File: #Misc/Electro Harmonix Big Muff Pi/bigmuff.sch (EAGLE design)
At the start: 33 parts, among them IC1 TL082CP, Q1 2N7000, Q2 2N7000

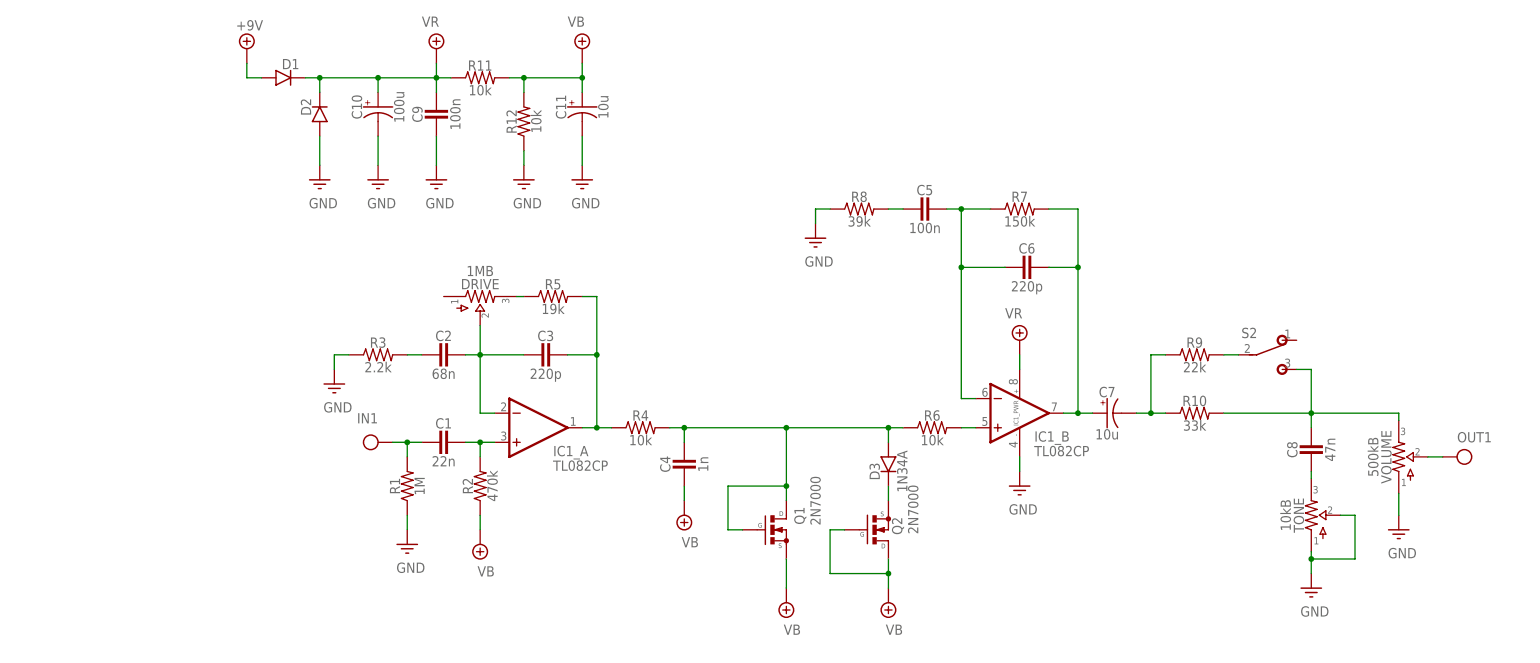
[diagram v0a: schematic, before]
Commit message: 20200322/09:12
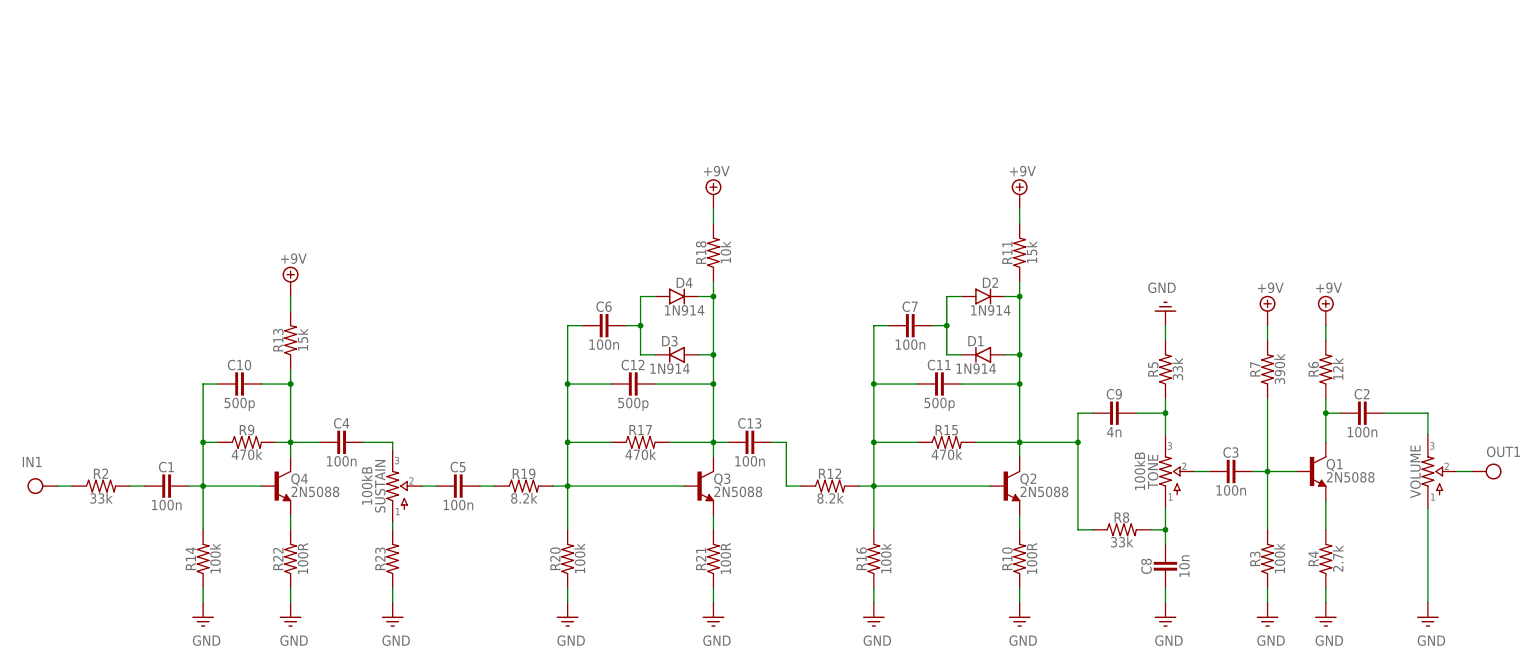
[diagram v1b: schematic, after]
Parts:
- removed DRIVE: 1MB, pedals-potentiometers:POTS16MM
- removed IC1: TL082CP, pedals-integrated circuits:DUALTH
- removed R1: 1M, pedals-resistors:R_.3B
- removed S2: (no value), pedals-switches:SPDT
- added C12: 500p, pedals-capacitors-film:CER/FILMBOX.1
- added C13: 100n, pedals-capacitors-film:CER/FILMBOX.1
- added D4: 1N914, pedals-diodes:DO41.2
- added Q3, Q4: 2N5088, pedals-transistors:2N5088
- added R13: 15k, pedals-resistors:R_.3B
- added R14, R16, R20: 100k, pedals-resistors:R_.3B
- added R15, R17: 470k, pedals-resistors:R_.3B
- added R18: 10k, pedals-resistors:R_.3B
- added R19: 8.2k, pedals-resistors:R_.3B
- added R21, R22: 100R, pedals-resistors:R_.3B
- added R23: (no value), pedals-resistors:R_.3B
- added SUSTAIN: 100kB, pedals-potentiometers:POTS16MM
- C1: value 22n -> 100n
- C10: value 100u -> 500p; device pedals-capacitors-elec:0500 -> pedals-capacitors-film:CER/FILMBOX.1
- C11: value 10u -> 500p; device pedals-capacitors-elec:0500 -> pedals-capacitors-film:CER/FILMBOX.1
- C2: value 68n -> 100n
- C3, C6: value 220p -> 100n
- C4: value 1n -> 100n
- C7: value 10u -> 100n; device pedals-capacitors-elec:0500 -> pedals-capacitors-film:CER/FILMBOX.1
- C8: value 47n -> 10n
- C9: value 100n -> 4n
- D1, D2: value (none) -> 1N914; device pedals-diodes:DO41.3 -> pedals-diodes:DO41.2
- D3: value 1N34A -> 1N914
- Q1, Q2: value 2N7000 -> 2N5088; device pedals-transistors:2N7000 -> pedals-transistors:2N5088
- R10: value 33k -> 100R
- R11: value 10k -> 15k
- R12: value 10k -> 8.2k
- R2: value 470k -> 33k
- R3: value 2.2k -> 100k
- R4: value 10k -> 2.7k
- R5: value 19k -> 33k
- R6: value 10k -> 12k
- R7: value 150k -> 390k
- R8: value 39k -> 33k
- R9: value 22k -> 470k
- TONE: value 10kB -> 100kB
- VOLUME: value 500kB -> (none)
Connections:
- removed net N$1: C7.-, R10.1, R9.1
- removed net N$15: R9.2, S2.P
- removed net N$8: C2.2, R3.2
- removed net VB: C11.+, C4.2, Q1.S, Q2.D, Q2.G, R11.2, R12.2, R2.1
- removed net VR: C10.+, C9.1, D1.C, D2.C, IC1_PWR.V+, R11.1
- new net N$18: C11.1, C9.2, D1.A, D2.C, Q2.C, R11.1, R15.2, R8.1
- new net N$19: C7.1, D1.C, D2.A
- new net N$2: C1.2, R2.2
- new net N$21: Q2.E, R10.2
- new net N$22: C3.2, TONE.2
- new net N$23: C9.1, R5.1, TONE.3
- new net N$24: C8.1, R8.2, TONE.1
- new net N$25: C3.1, Q1.B, R3.2, R7.1
- new net N$29: C2.2, Q1.C, R6.1
- new net N$3: C1.1, C10.2, Q4.B, R14.2, R9.1
- new net N$30: C2.1, VOLUME.3
- new net N$32: Q1.E, R4.2
- net +9V: now also R11.2, R13.2, R18.2, R6.2, R7.2; no longer D1.A
- net GND: now also C8.2, R10.1, R14.1, R16.1, R20.1, R21.1, R22.1, R23.1, R4.1, R5.2; no longer C10.-, C11.-, C9.2, D2.A, IC1_PWR.V-, R1.1, R12.1, R8.1, TONE.1, TONE.2
- net IN: now also R2.1; no longer C1.2, R1.2
- net N$10: now also C5.1, R19.1; no longer D3.C, Q2.S
- net N$11: now also C12.2, C6.2, Q3.B, R17.1, R19.2, R20.2; no longer C4.1, D3.A, Q1.D, Q1.G, R4.2, R6.1
- net N$12: now also C12.1, C13.2, D3.A, D4.C, Q3.C, R17.2, R18.1; no longer C5.1, C6.2, IC1_B.-IN, R7.1
- net N$13: now also Q3.E, R21.2; no longer C6.1, C7.+, IC1_B.OUT, R7.2
- net N$14: now also C6.1, D3.C, D4.A; no longer C5.2, R8.2
- net N$16: now also C13.1, R12.1; no longer C8.1, R10.2, S2.S, VOLUME.3
- net N$17: now also C11.2, C7.2, Q2.B, R12.2, R15.1, R16.2; no longer C8.2, TONE.3
- net N$4: now also Q4.E, R22.2; no longer C1.1, IC1_A.+IN, R2.2
- net N$5: now also C10.1, C4.2, Q4.C, R13.1, R9.2; no longer C2.1, C3.2, DRIVE.2, IC1_A.-IN
- net N$6: now also C4.1, SUSTAIN.3; no longer DRIVE.3, R5.1
- net N$7: now also R23.2, SUSTAIN.1; no longer C3.1, IC1_A.OUT, R4.1, R5.2
- net N$9: now also C5.2, SUSTAIN.2; no longer IC1_B.+IN, R6.2
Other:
- moved on the sheet: C1, C2, C3, C4, C5, C6, C8, C9, D1, D2, D3, R10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
